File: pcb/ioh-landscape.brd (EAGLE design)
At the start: 50.8 x 81.3 mm, 35 parts

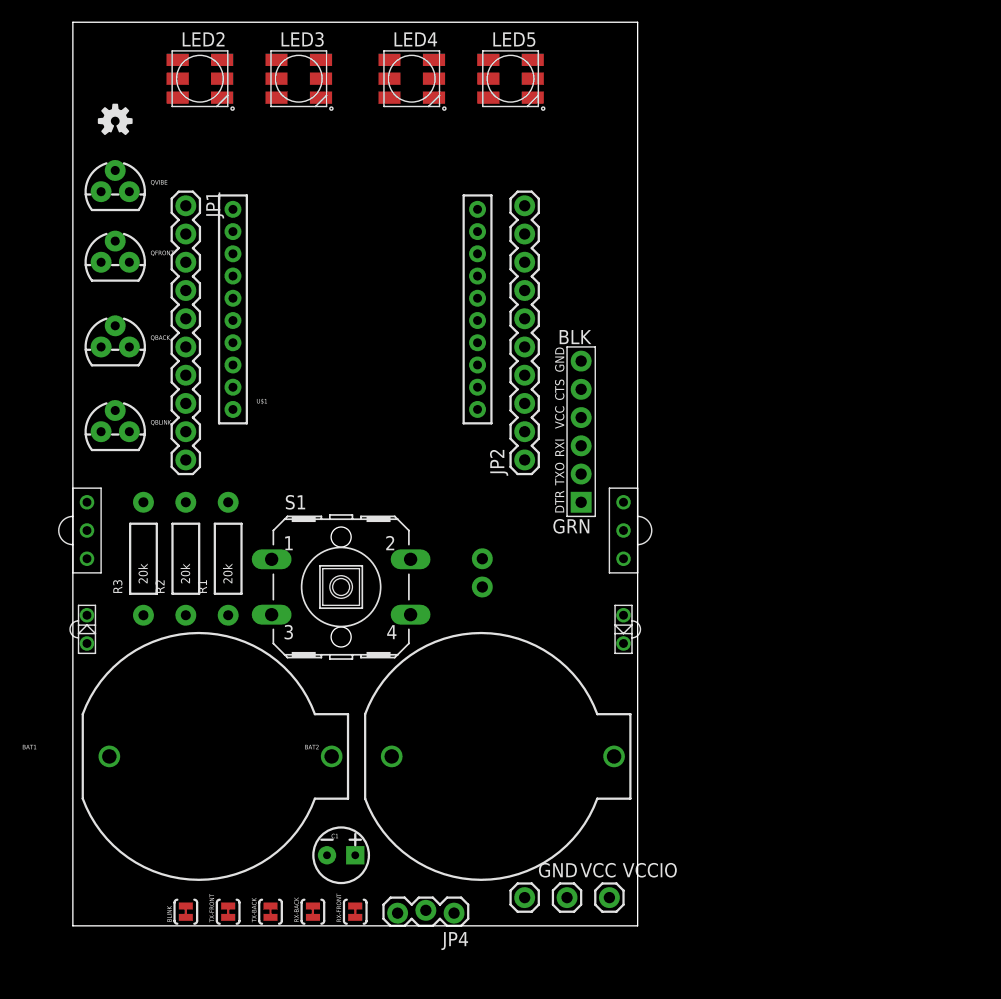
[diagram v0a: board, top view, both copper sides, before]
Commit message: playing around with layouts
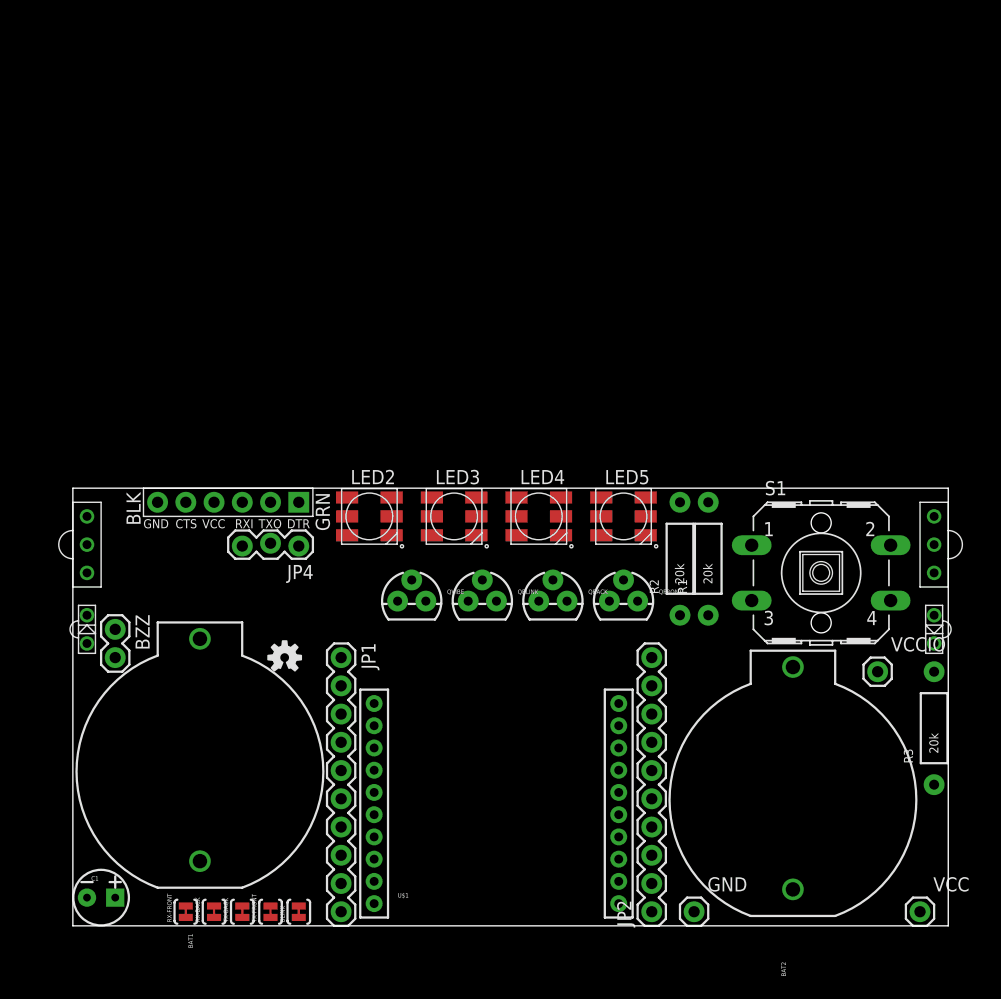
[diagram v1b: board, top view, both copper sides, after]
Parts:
- moved R3 72.7 mm to (77.5, 17.8)
- moved U$2 66.3 mm to (2.54, 26.7), turned to 0 degrees
- moved QFRONT 54.9 mm to (49.5, 29.2)
- moved LOGO1 50.6 mm to (19.1, 24.1)
- moved U$1 46.2 mm to (38.1, 11.4)
- moved QBACK 45.5 mm to (43.2, 29.2)
- moved QVIBE 45.5 mm to (30.5, 29.2)
- moved R2 44.5 mm to (54.6, 33.0)
- moved S1 43.2 mm to (67.3, 31.8)
- moved R1 43.2 mm to (57.1, 33.0)
- moved JP1 43.0 mm to (24.1, 24.1)
- moved LED2 42.2 mm to (26.7, 36.8)
- moved JP2 42.2 mm to (52.1, 1.27)
- moved LED3 41.8 mm to (34.3, 36.8)
- moved LED4 41.0 mm to (41.9, 36.8)
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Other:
- board size 50.8 x 81.3 mm -> 78.7 x 39.4 mm
